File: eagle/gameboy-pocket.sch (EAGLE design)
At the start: 33 parts, among them J1 AUDIO_JACK_3.5MM_PTH, U1 LM4875

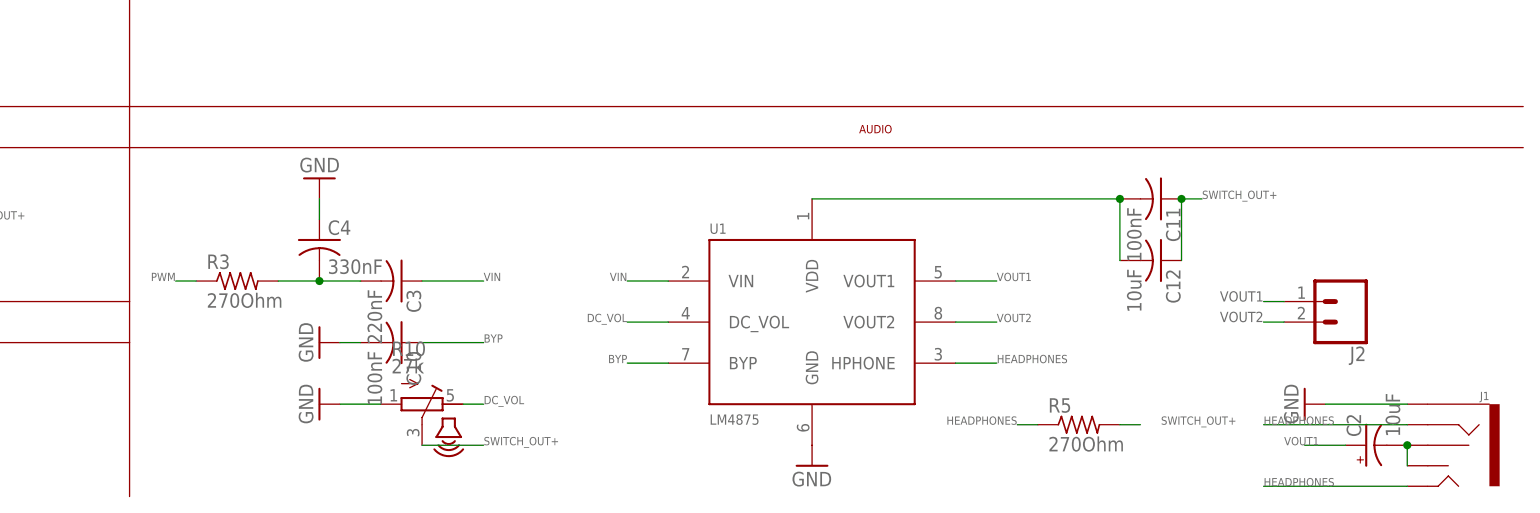
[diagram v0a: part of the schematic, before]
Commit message: Wed 21 Feb 2018 12:43:42 EST
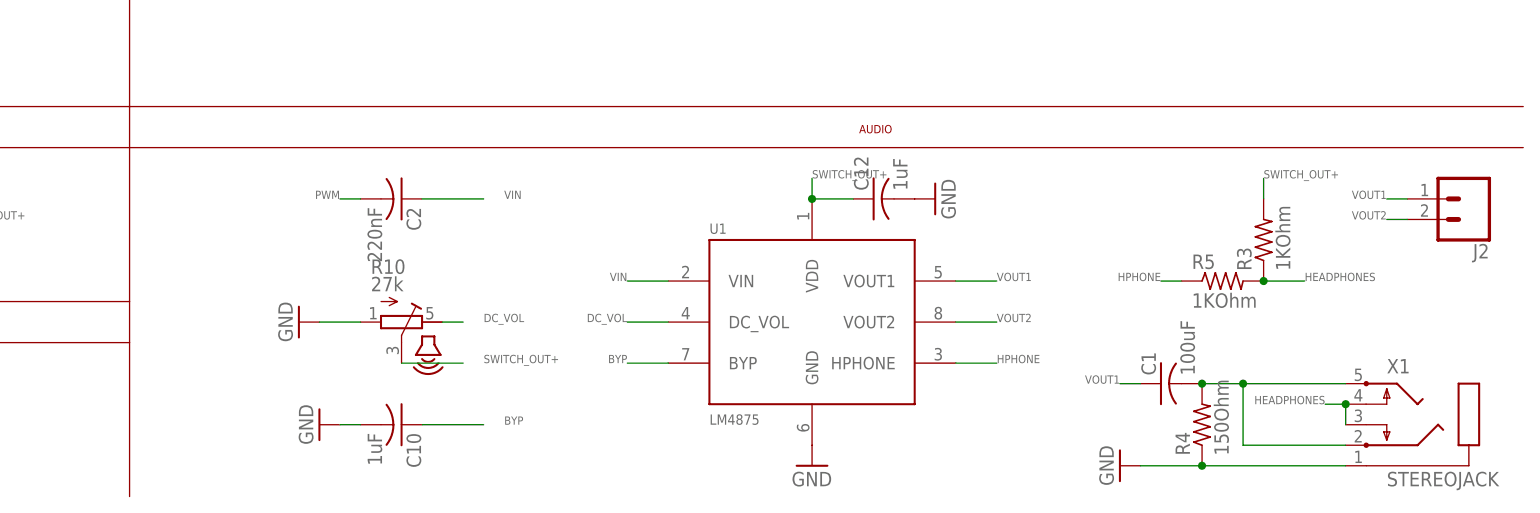
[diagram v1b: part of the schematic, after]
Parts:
- removed C11: 100nF, adafruit:C-USC0805
- removed C3: 220nF, adafruit:C-USC0805
- removed C4: 330nF, adafruit:C-USC0805
- removed J1: AUDIO_JACK_3.5MM_PTH, SparkFun-Connectors:AUDIO_JACK_3.5MM_PTH
- added C1: 100uF, adafruit:C-USC0805
- added R4: 150Ohm, adafruit:R-US_R0805
- added X1: STEREOJACK, adafruit:STEREOJACK
- C10: value 100nF -> 1uF
- C12: value 10uF -> 1uF
- C2: value 10uF -> 220nF; device SparkFun-Capacitors:10UF-POLAR-EIA3216-16V-10%(TANT) -> adafruit:C-USC0805
- R3, R5: value 270Ohm -> 1KOhm
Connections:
- removed net CAP_LINE: C11.2, C12.2, U1.VDD
- removed net CAP_LINE_JACK: C2.-, J1.RSH, J1.TSH
- removed net N$2: C3.2, C4.2, R3.2
- new net HPHONE: R5.1, U1.HPHONE
- new net VIN1: C1.2, R4.2, X1.2, X1.5
- net GND: now also C12.2, R4.1, X1.1; no longer C4.1, J1.SLEEVE
- net HEADPHONES: now also R3.1, R5.2, X1.3, X1.4; no longer J1.RING, J1.TIP, R5.1, U1.HPHONE
- net PWM: now also C2.2; no longer R3.1
- net SWITCH_OUT+: now also R3.2, U1.VDD; no longer C11.1, R5.2
- net VIN: now also C2.1; no longer C3.1
- net VOUT1: now also C1.1; no longer C2.+
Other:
- moved on the sheet: C10, C12, J2, R10, R3, R5
